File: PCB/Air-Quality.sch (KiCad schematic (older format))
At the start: 17 parts, among them J1 Conn_01x07_Female, SW1 SW_Push, SW2 SW_SPST, U1 Pico

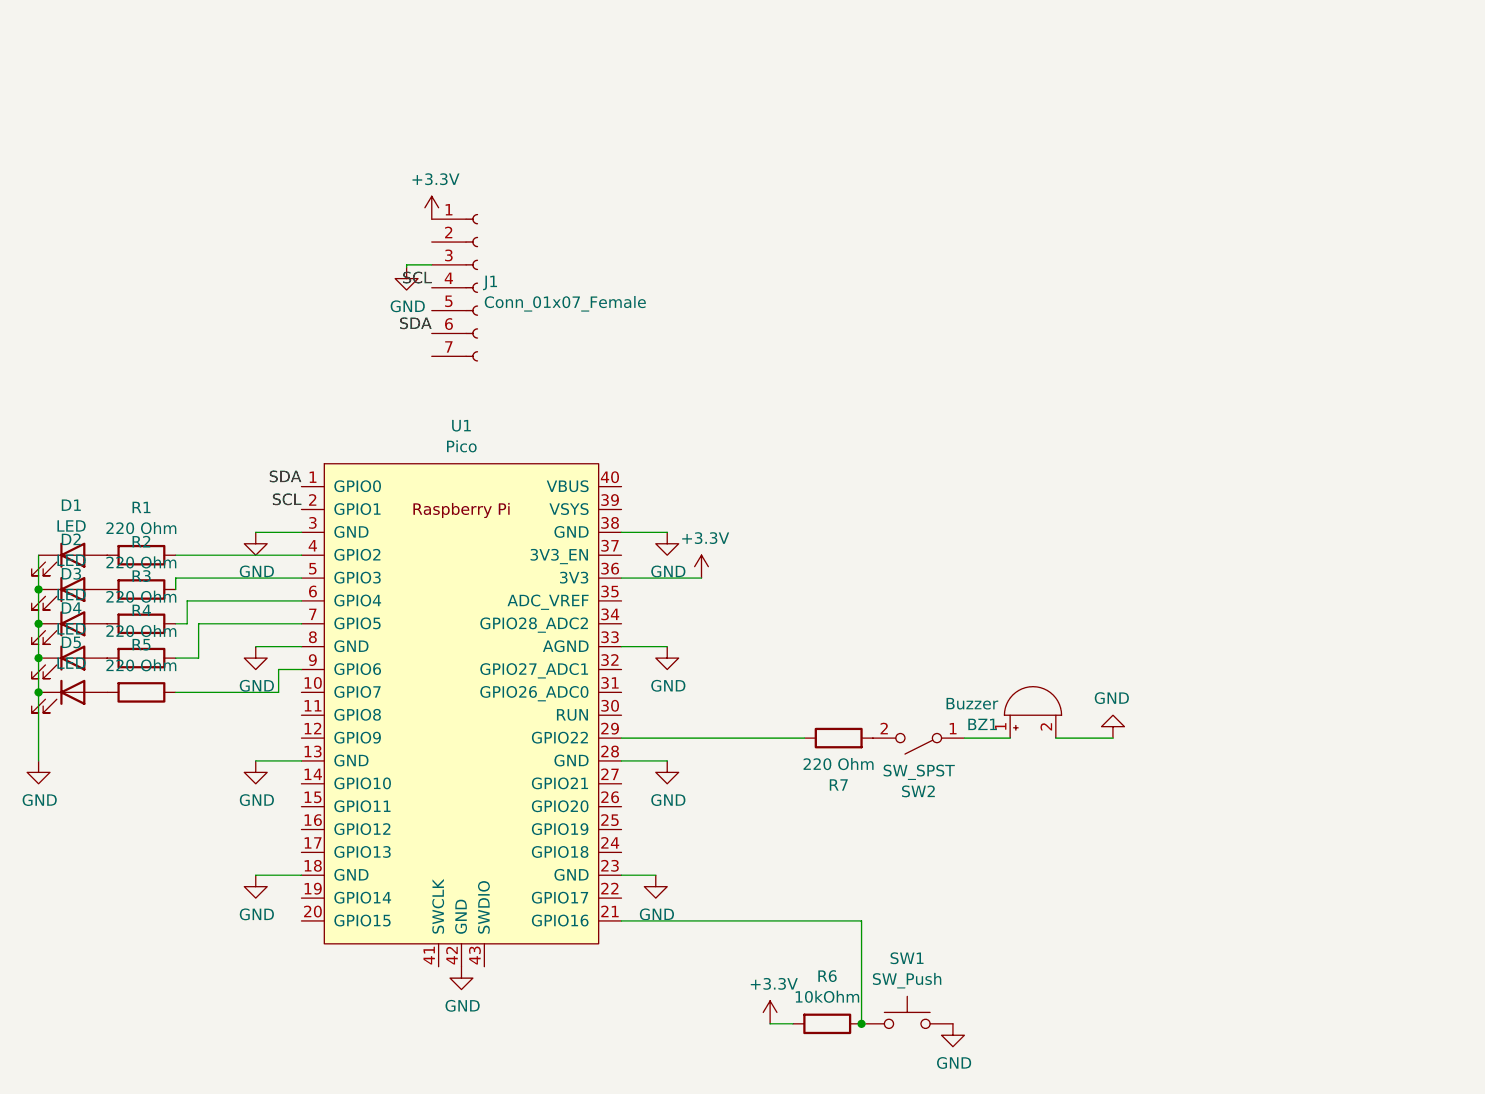
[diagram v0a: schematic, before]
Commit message: Version 3 for friends.
Seeeduino
New Sensor
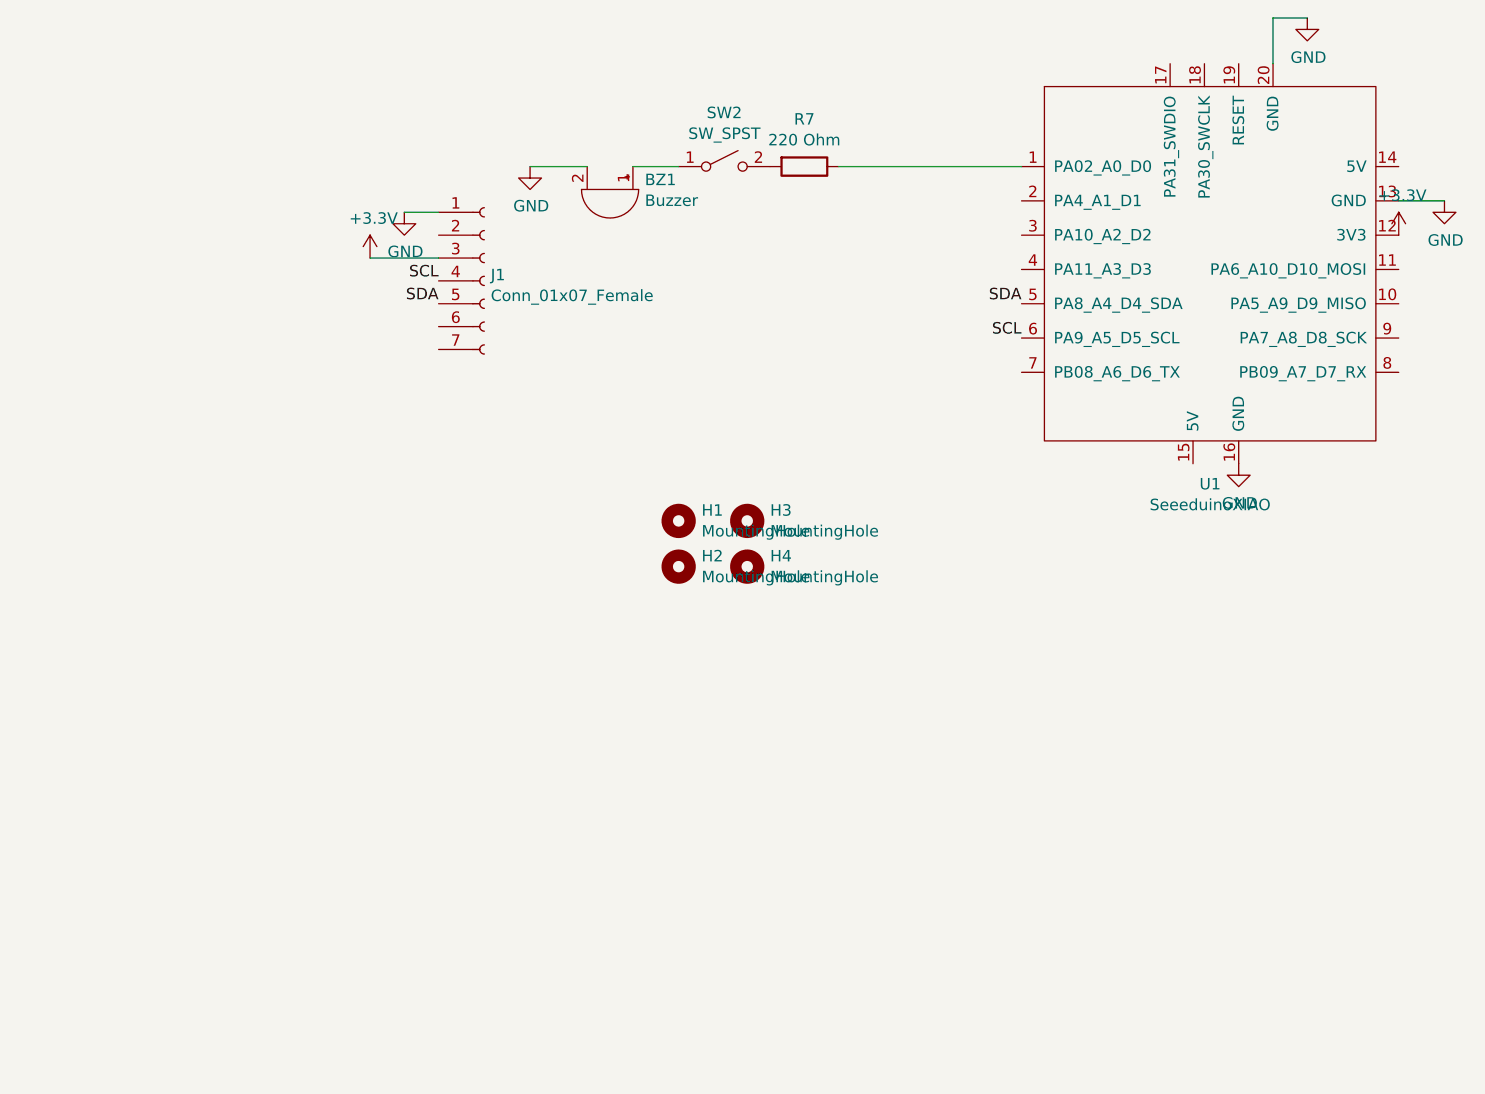
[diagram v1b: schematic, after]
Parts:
- removed D1, D2, D3, D4, D5: LED, LED_SMD:LED_0805_2012Metric, symbol Device:LED
- removed R1, R2, R3, R4, R5: 220 Ohm, Resistor_SMD:R_0805_2012Metric, symbol Device:R
- removed R6: 10kOhm, Resistor_SMD:R_0805_2012Metric, symbol Device:R
- removed SW1: SW_Push, Button_Switch_THT:SW_PUSH_6mm, symbol Switch:SW_Push
- removed U1: Pico, MCU_RaspberryPI_and_Board:RPi_Pico_SMD_TH, symbol RaspberryPi_and_Board:Pico
- added H1, H2, H3, H4: MountingHole, MountingHole:MountingHole_2.7mm_M2.5_ISO14580, symbol Mechanical:MountingHole
- added U1: SeeeduinoXIAO, Seeeduino XIAO KICAD:Seeeduino XIAO-MOUDLE14P-2.54-21X17.8MM, symbol Seeeduino_XIAO:SeeeduinoXIAO
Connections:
- net +3V3: now also J1.3 (Pin_3), U1.12 (3V3); no longer J1.1 (Pin_1)
- net GND: now also J1.1 (Pin_1), U1.13 (GND), U1.16 (GND), U1.20 (GND); no longer J1.3 (Pin_3)
- net SCL: now also U1.6 (PA9_A5_D5_SCL)
- net SDA: now also J1.5 (Pin_5), U1.5 (PA8_A4_D4_SDA); no longer J1.6 (Pin_6)
- net at R7.1: now also U1.1 (PA02_A0_D0)
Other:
- moved on the sheet: BZ1, J1, R7, SW2
